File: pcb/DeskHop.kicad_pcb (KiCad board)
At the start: 2 copper layers, 66.9 x 74.5 mm, 12 parts, among them J1 Keyboard In, J2 Debug2, J3 Debug1, J4 Mouse In, U1 Pico Primary, U2 Pico Secondary, U4 ADuM1201BR

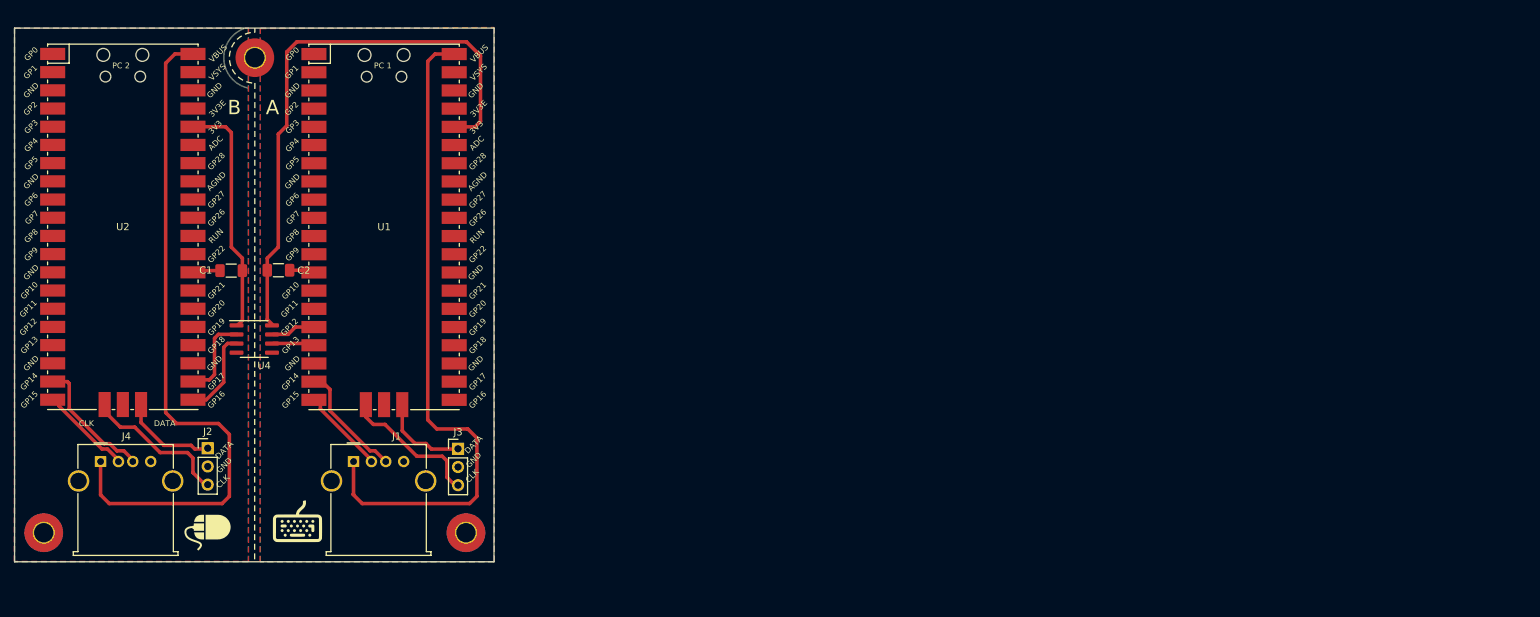
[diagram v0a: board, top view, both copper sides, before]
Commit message: bs changes
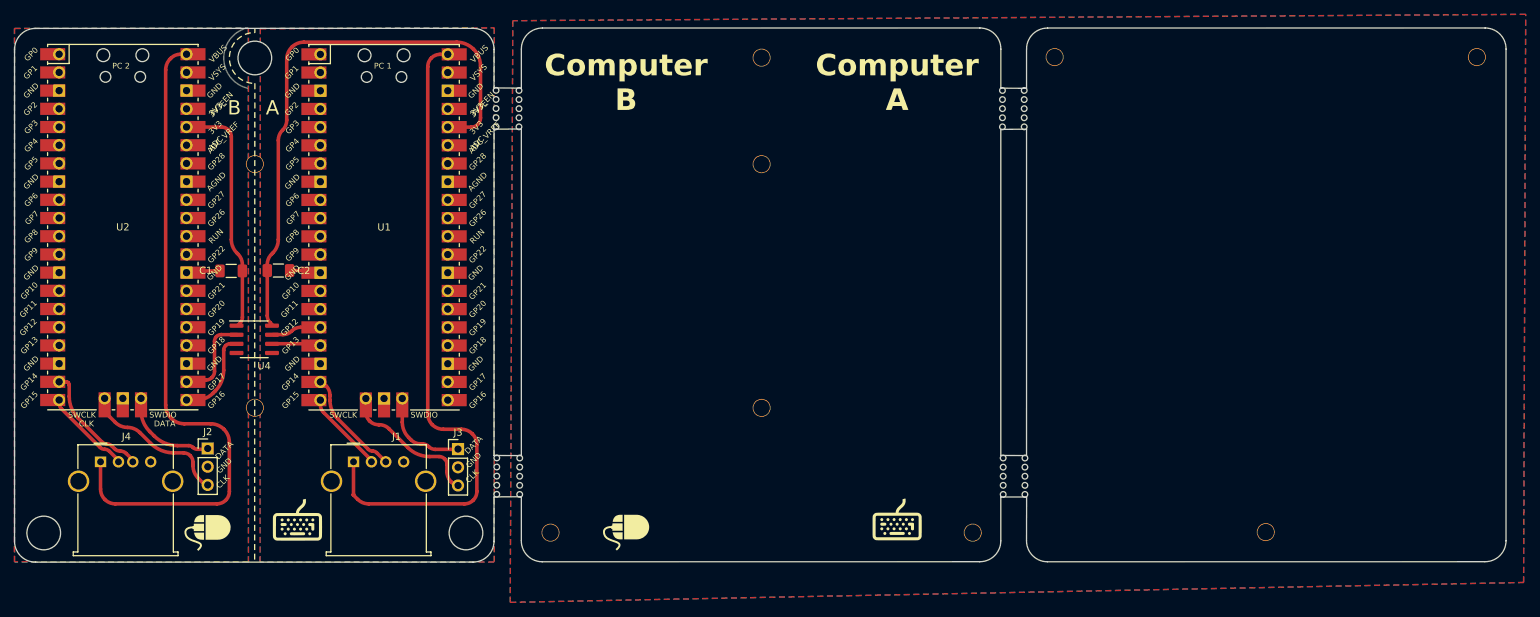
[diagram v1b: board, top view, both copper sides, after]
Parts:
- added G***: r, bs_custom_kicad:bs_logo_new_40mm, F.Cu at (138.0, 78.3)
- added H1: MountingHole_Pad, bs_custom_kicad:MountingHole_M2-clean, F.Cu at (67.3, 94.1)
- added H1: MountingHole_Pad, bs_custom_kicad:MountingHole_M2-clean, F.Cu at (138.0, 94.1)
- added H1: MountingHole_Pad, bs_custom_kicad:MountingHole_M2-clean, F.Cu at (67.3, 60.1)
- added H1: MountingHole_Pad, bs_custom_kicad:MountingHole_M2-clean, F.Cu at (237.9, 45.1)
- added H1: MountingHole_Pad, bs_custom_kicad:MountingHole_M2-clean, F.Cu at (138.0, 60.1)
- added H1: MountingHole_Pad, bs_custom_kicad:MountingHole_M2-clean, F.Cu at (108.6, 111.5)
- added H2: MountingHole_Pad, bs_custom_kicad:MountingHole_M2-clean, F.Cu at (178.9, 45.1)
- added H2: MountingHole_Pad, bs_custom_kicad:MountingHole_M2-clean, F.Cu at (167.5, 111.5)
- added H3: MountingHole_Pad, bs_custom_kicad:MountingHole_M2-clean, F.Cu at (138.0, 45.2)
- added H3: MountingHole_Pad, bs_custom_kicad:MountingHole_M2-clean, F.Cu at (208.4, 111.4)
- added REF**: breakaway-mousebites, Keebio-Parts:breakaway-mousebites, F.Cu at (174.9, 52.3)
- added REF**: breakaway-mousebites, Keebio-Parts:breakaway-mousebites, F.Cu at (175.0, 103.6)
- added REF**: breakaway-mousebites, Keebio-Parts:breakaway-mousebites, F.Cu at (171.4, 52.3)
- added REF**: breakaway-mousebites, Keebio-Parts:breakaway-mousebites, F.Cu at (171.5, 103.6)
- added REF**: breakaway-mousebites, Keebio-Parts:breakaway-mousebites, F.Cu at (104.5, 103.6)
- added REF**: breakaway-mousebites, Keebio-Parts:breakaway-mousebites, F.Cu at (104.4, 52.3)
- added REF**: breakaway-mousebites, Keebio-Parts:breakaway-mousebites, F.Cu at (100.8, 103.6)
- added REF**: breakaway-mousebites, Keebio-Parts:breakaway-mousebites, F.Cu at (100.7, 52.3)
- H1, H2: footprint MountingHole:MountingHole_2.7mm_M2.5_Pad_TopBottom -> bs_custom_kicad:pcb stand off hole
- H3: footprint MountingHole:MountingHole_2.7mm_M2.5_Pad_TopOnly -> bs_custom_kicad:pcb stand off hole
- U1, U2: footprint MCU_RaspberryPi_and_Boards:RPi_Pico_SMD_Nohole -> MCU_RaspberryPi_and_Boards:RPi_Pico_SMD_TH
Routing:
- net Net-(U1-3V3): track 82.1 -> 80.9 mm
- net Net-(J4-VBUS): track 94.6 -> 93.5 mm
- net Net-(J1-VBUS): track 91.9 -> 91.0 mm
- net Net-(J2-Pin_3): track 21.4 -> 20.6 mm
- net Net-(J3-Pin_3): track 19.6 -> 18.9 mm
- net Net-(J2-Pin_1): track 14.0 -> 13.5 mm
- added copper zone on B.Cu, net (none)
- added copper zone on F.Cu, net (none)
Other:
- board size 66.9 x 74.5 mm -> 208.2 x 74.5 mm
- board text added: "Computer A"
- board text added: "Computer B"
